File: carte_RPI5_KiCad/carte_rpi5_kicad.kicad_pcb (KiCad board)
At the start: 2 copper layers, 153.6 x 69 mm, 29 parts, among them J10 RPI5_40pins, J12 XT60-M

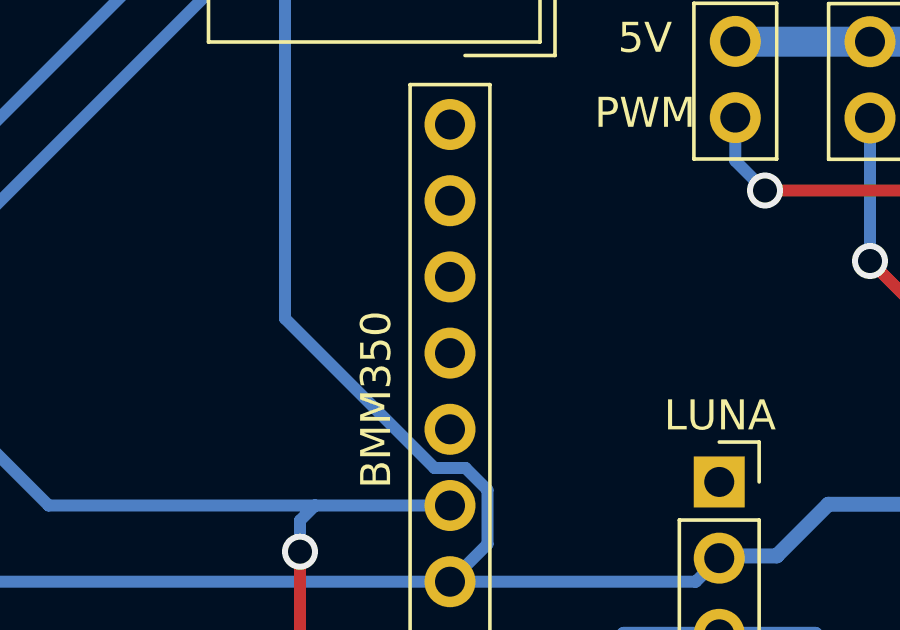
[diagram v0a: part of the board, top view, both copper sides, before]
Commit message: modif2_carte_dirigeable
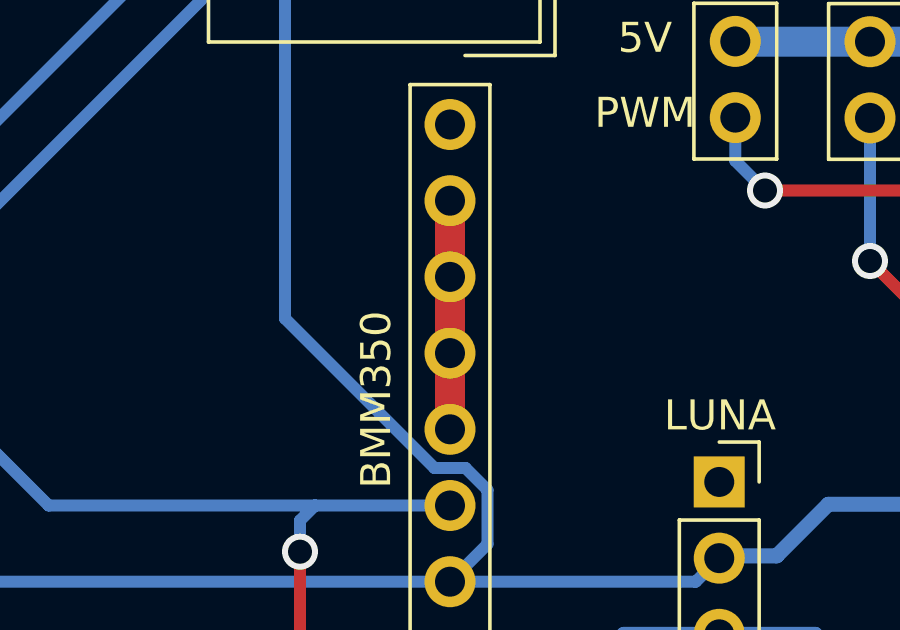
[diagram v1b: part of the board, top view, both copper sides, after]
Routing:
- net NC: track 0.00 -> 7.62 mm
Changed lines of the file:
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@@
 		(net "PWM6")
+	)
+	(segment
+		(start 70 82.84)
+		(end 70 90.46)
+		(width 1)
+		(layer "F.Cu")
+		(net "NC")
 	)
 	(zone
